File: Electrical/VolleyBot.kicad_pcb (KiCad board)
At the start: 2 copper layers, 80 x 52 mm, 77 parts, among them J1 Conn_01x04_Pin, J2 Conn_01x04_Pin, J3 Conn_01x02_Socket, J4 Conn_01x04_Socket, J5 Conn_01x02_Socket, J6 Conn_01x02_Socket, J7 Conn_01x02_Socket, Q1 AO3401A, Q2 AO3401A, SW1 SW_SPDT, SW2 SW_SPDT, SW3 SW_SPDT, U1 STM32F411CEU6, U2 DRV8833PWP, U3 DRV8833PWP, U4 AP62300TWU, U5 AP62300TWU, Y1 16MHz

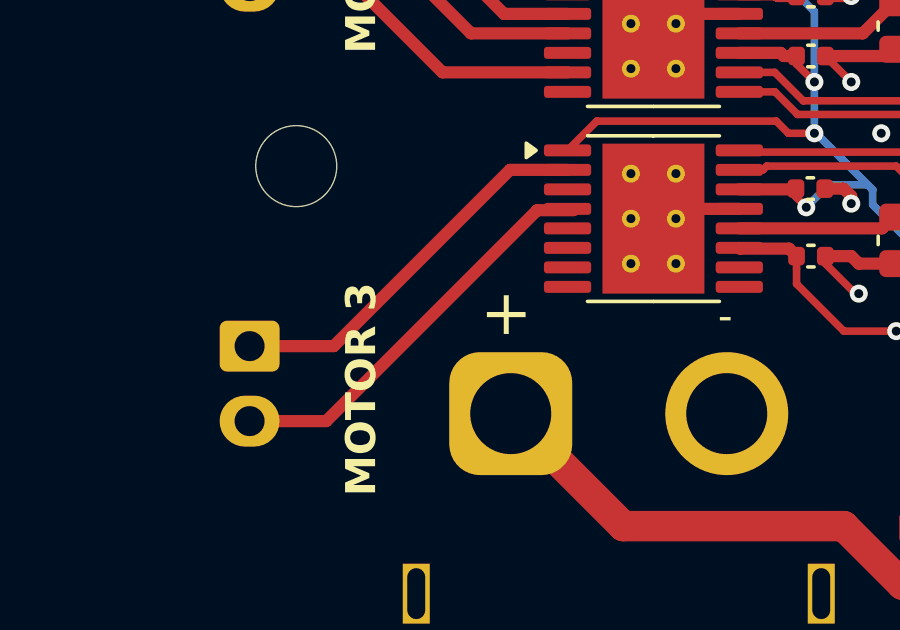
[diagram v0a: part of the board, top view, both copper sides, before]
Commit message: update
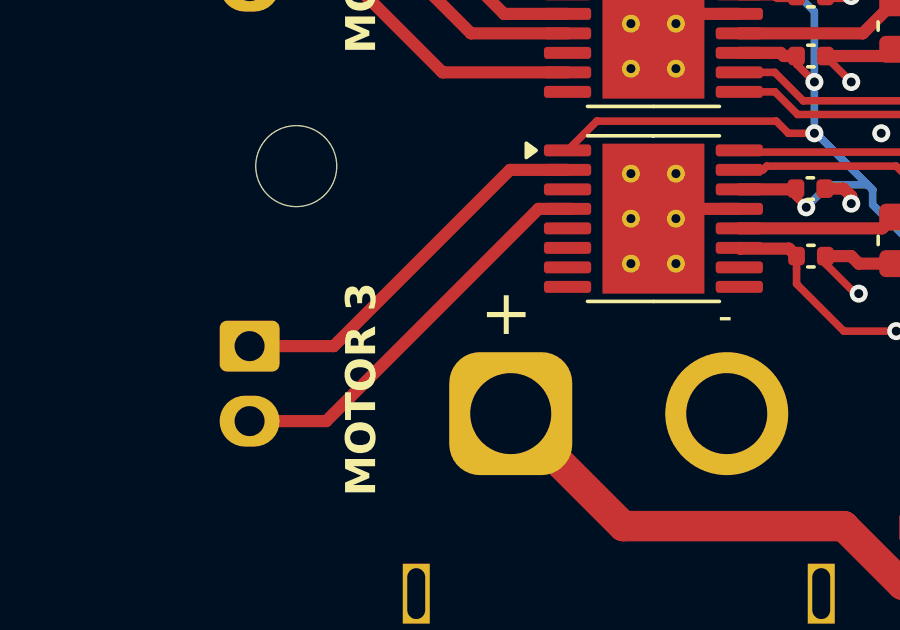
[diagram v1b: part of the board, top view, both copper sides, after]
